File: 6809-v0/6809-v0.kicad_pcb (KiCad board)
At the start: 2 copper layers, 2 parts, among them U1 MC68B09

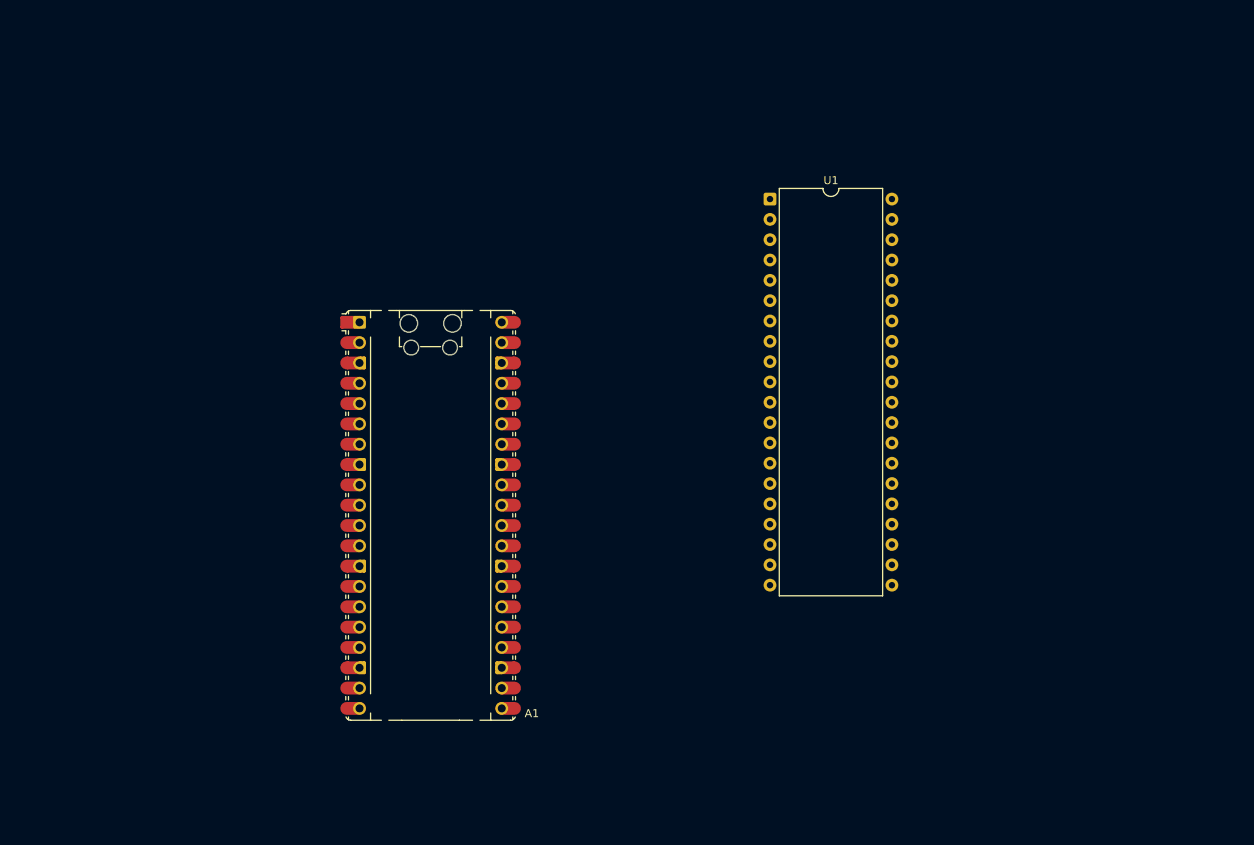
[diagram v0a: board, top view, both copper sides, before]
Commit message: First checking of 6809 board:
- KiCad 9.0.5
- prior to upgrade
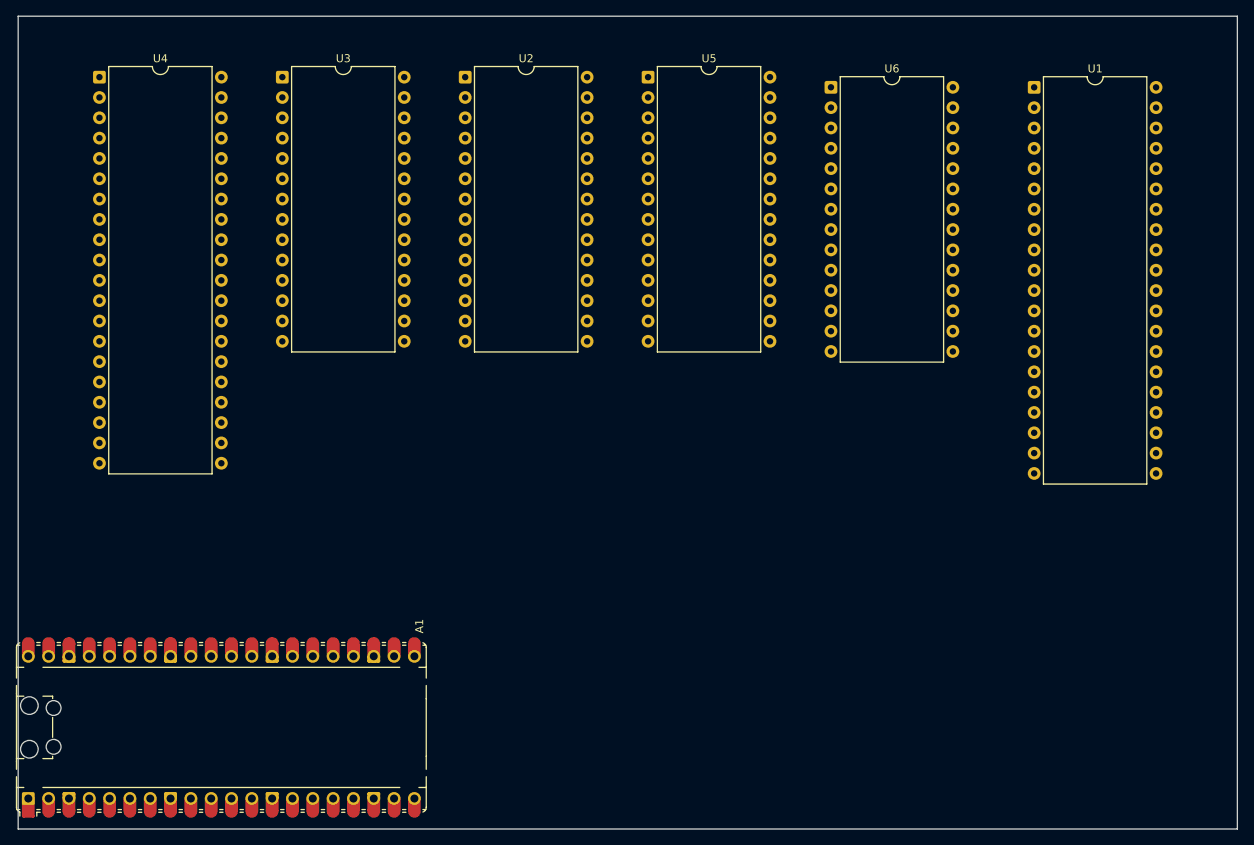
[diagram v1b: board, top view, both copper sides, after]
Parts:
- added U2: 2764, Package_DIP:DIP-28_W15.24mm, F.Cu at (91.4, 35.6)
- added U3: W65C51NxP, Package_DIP:DIP-28_W15.24mm, F.Cu at (68.6, 35.6)
- added U4: W65C22NxP, Package_DIP:DIP-40_W15.24mm, F.Cu at (45.7, 35.6)
- added U5: CY62256-70PC, Package_DIP:DIP-28_W15.24mm, F.Cu at (114.3, 35.6)
- added U6: CY62256-70PC, Package_DIP:DIP-28_W15.24mm, F.Cu at (137.2, 36.8)
- moved A1 37.2 mm to (61.0, 116.8), turned to 90 degrees
- moved U1 35.9 mm to (162.6, 36.8)
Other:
- board outline added: 152.4 x 101.6 mm
